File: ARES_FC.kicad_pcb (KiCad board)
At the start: 2 copper layers, 57.2 x 57.2 mm, 67 parts, among them J1 SWD, J2 TYPE-C-31-M-12, J3 FC_M/P, J4 5V, J5 GND, J6 FC_RF, J7 Conn_01x04_Pin, J8 Conn_01x04_Pin, U1 STM32F401CCU6, U2 AMS1117-3.3, U3 BMP280, U4 BNO055, U5 W25Q32JVSS, U6 PA1616S, Y1 16MHz, Y2 32.768kHz

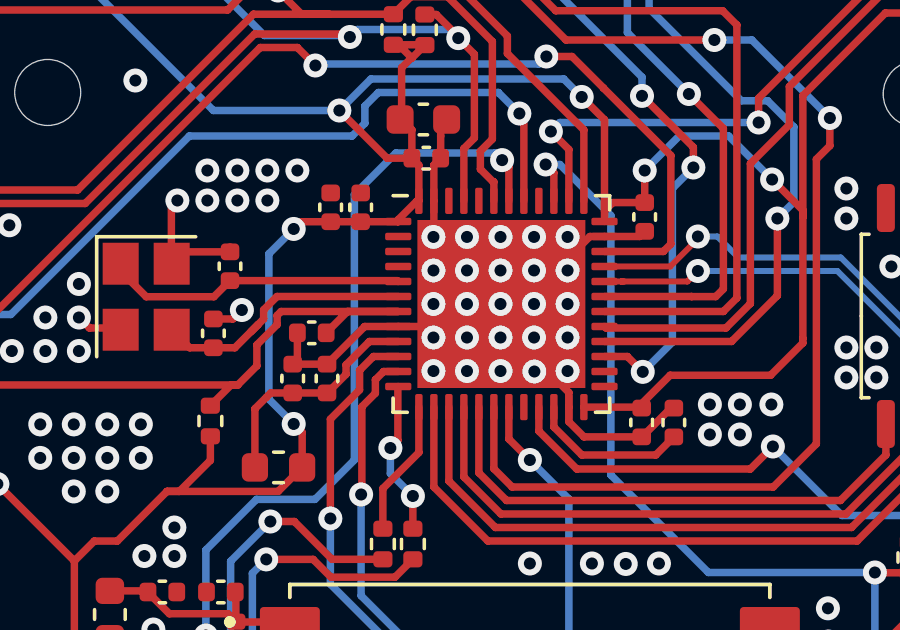
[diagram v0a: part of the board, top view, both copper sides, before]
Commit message: added gerbers & CPL for ordering
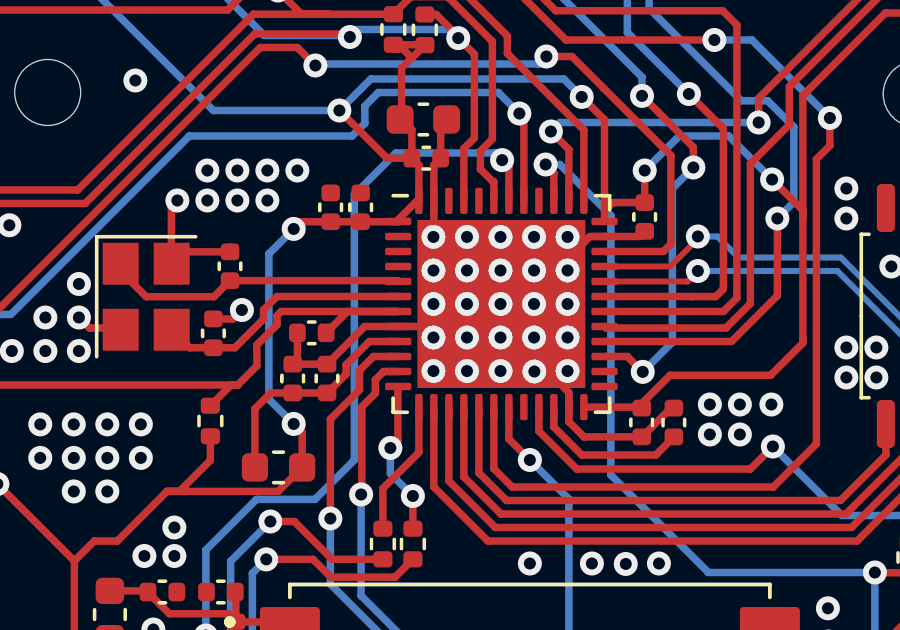
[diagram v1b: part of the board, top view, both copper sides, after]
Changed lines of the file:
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@@
 			(plot_on_all_layers_selection 0x0000000_00000000)
 			(disableapertmacros no)
-			(usegerberextensions no)
-			(usegerberattributes yes)
-			(usegerberadvancedattributes yes)
-			(creategerberjobfile yes)
+			(usegerberextensions yes)
+			(usegerberattributes no)
+			(usegerberadvancedattributes no)
+			(creategerberjobfile no)
 			(dashed_line_dash_ratio 12.000000)
 			(dashed_line_gap_ratio 3.000000)
@@
 			(psa4output no)
 			(plotreference yes)
-			(plotvalue yes)
+			(plotvalue no)
 			(plotfptext yes)
 			(plotinvisibletext no)
 			(sketchpadsonfab no)
-			(subtractmaskfromsilk no)
+			(subtractmaskfromsilk yes)
 			(outputformat 1)
 			(mirror no)
@@
 				(font
 					(size 1.27 1.27)
+					(thickness 0.15)
 				)
 			)
@@
 				(font
 					(size 1.27 1.27)
+					(thickness 0.15)
 				)
 			)
@@
 				(font
 					(size 1.27 1.27)
+					(thickness 0.15)
 				)
 			)
@@
 	)
 	(segment
-		(start 142.487653 92.737653)
-		(end 142.675 92.550305)
+		(start 147.1625 91.79974)
+		(end 143.12029 91.79974)
 		(width 0.25)
 		(layer "F.Cu")
@@
 	)
 	(segment
-		(start 141.716766 93.50854)
-		(end 142.487653 92.737653)
+		(start 142.675 92.550305)
+		(end 141.716765 93.50854)
 		(width 0.25)
 		(layer "F.Cu")
@@
 	)
 	(segment
-		(start 143.12029 91.79974)
-		(end 147.1625 91.79974)
+		(start 141.716765 93.50854)
+		(end 141 93.50854)
 		(width 0.25)
 		(layer "F.Cu")
@@
 	(segment
 		(start 142.675 92.24503)
-		(end 143.12029 91.79974)
-		(width 0.25)
-		(layer "F.Cu")
-		(net 4)
-	)
-	(segment
-		(start 141 93.50854)
-		(end 141.716766 93.50854)
+		(end 142.675 92.550305)
 		(width 0.25)
 		(layer "F.Cu")
@@
 	)
 	(segment
-		(start 142.675 92.550305)
+		(start 143.12029 91.79974)
 		(end 142.675 92.24503)
 		(width 0.25)
@@
 	)
 	(segment
-		(start 142.250305 92.975)
-		(end 142.487653 92.737653)
-		(width 0.25)
-		(layer "F.Cu")
-		(net 4)
-	)
-	(segment
 		(start 142.65 79.2)
 		(end 145.375 76.475)
@@
 	)
 	(segment
+		(start 156.80026 91.29974)
+		(end 154.0375 91.29974)
+		(width 0.2)
+		(layer "F.Cu")
+		(net 13)
+	)
+	(segment
 		(start 171.2625 99.53)
 		(end 171.2625 100.07)
@@
 	)
 	(segment
-		(start 154.6 91.29974)
-		(end 154.693751 91.29974)
-		(width 0.2)
-		(layer "F.Cu")
-		(net 13)
-	)
-	(segment
-		(start 154.0375 91.29974)
-		(end 154.6 91.29974)
-		(width 0.2)
-		(layer "F.Cu")
-		(net 13)
-	)
-	(segment
-		(start 156.80026 91.29974)
-		(end 154.6 91.29974)
-		(width 0.2)
-		(layer "F.Cu")
-		(net 13)
-	)
-	(segment
 		(start 171.2625 100.07)
 		(end 171.4925 100.3)
@@
 	)
 	(segment
-		(start 157.15 90.95)
-		(end 156.80026 91.29974)
-		(width 0.2)
-		(layer "F.Cu")
-		(net 13)
-	)
-	(segment
 		(start 170.15 99.3)
 		(end 172.3125 99.3)
@@
 		(width 0.2)
 		(layer "F.Cu")
+		(net 13)
+	)
+	(segment
+		(start 157.15 90.95)
+		(end 156.80026 91.29974)
+		(width 0.2)
+		(layer "F.Cu")
